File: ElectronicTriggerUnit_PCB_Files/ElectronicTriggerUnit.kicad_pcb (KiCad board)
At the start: 2 copper layers, 59.7 x 50 mm, 50 parts, among them IC1 MCP1407-E_SN, IC2 ATTINY814-SSF, J2 Conn_01x05, J4 Conn_01x04, Q1 LC191PTDT, Q2 LKPT30102B-A01, Q3 78-SQRS140ELP, Q4 LC191PTDT, U1 Gnd, U2 12v, U3 GndMotor, U4 Gnd, U5 12v

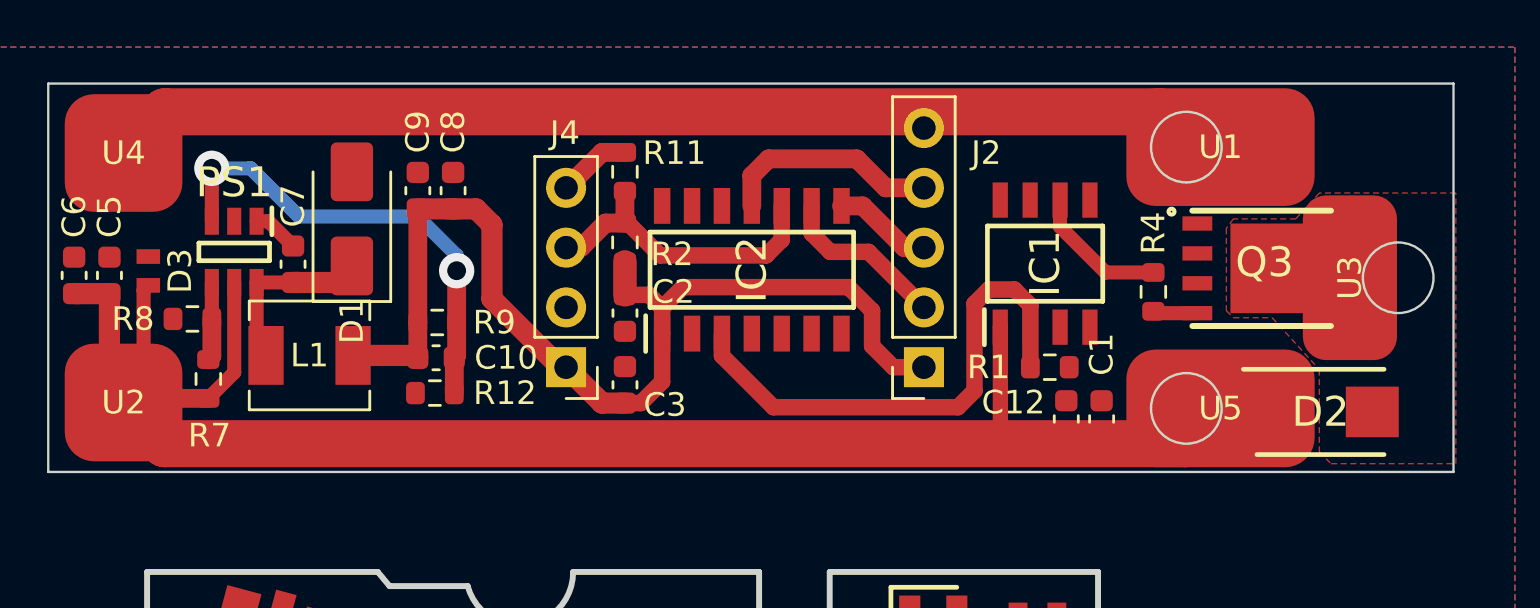
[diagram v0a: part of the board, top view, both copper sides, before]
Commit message: Fixes
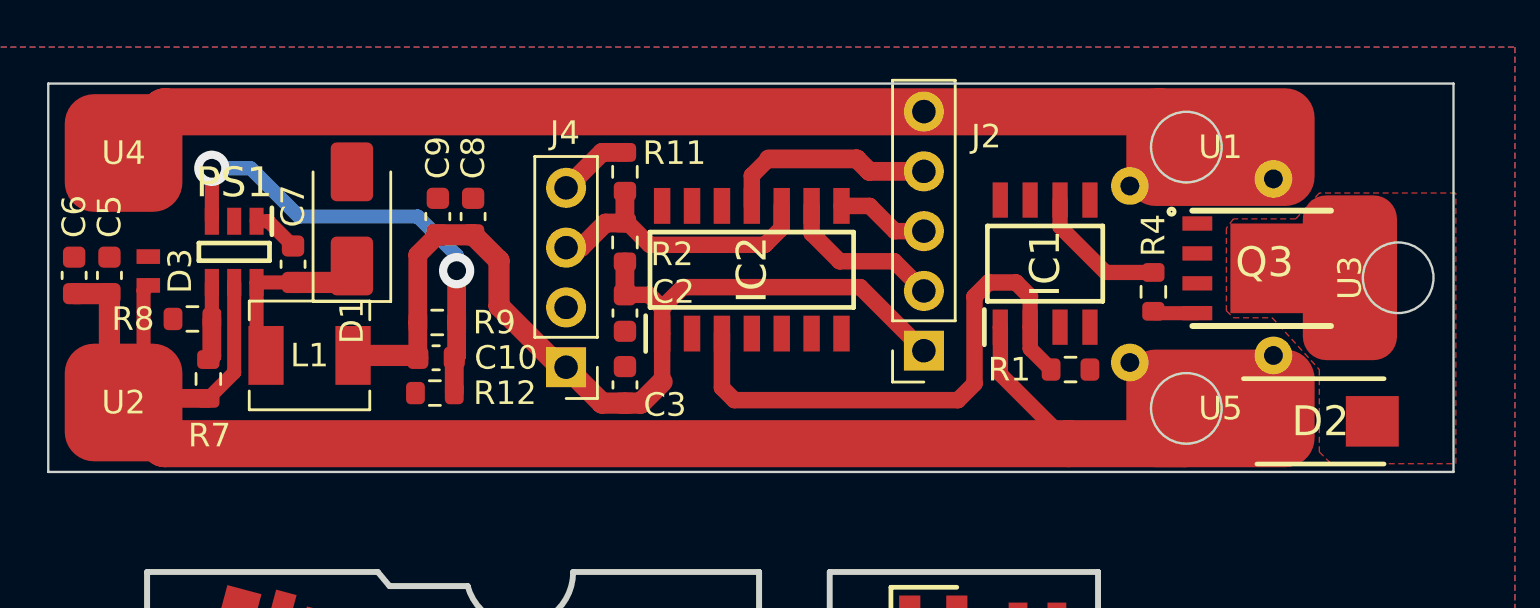
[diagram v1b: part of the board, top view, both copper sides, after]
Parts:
- C1, C12: footprint Capacitor_SMD:C_0603_1608Metric -> Capacitor_THT:C_Axial_L5.1mm_D3.1mm_P7.50mm_Horizontal; moved to B.Cu
- moved C1 9.97 mm to (110.6, 83.4)
- moved C12 9.20 mm to (116.7, 90.6)
- moved C8 1.39 mm to (82.7, 84.7)
- moved C9 1.39 mm to (81.2, 84.7)
- moved R1 0.89 mm to (108.1, 91.2)
- moved J2 0.70 mm to (101.8, 90.4)
- moved D2 0.40 mm to (118.7, 93.4)
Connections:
- LED4 pad 3: GND -> (no net)
- Q2 pad 3: GND -> (no net)
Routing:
- net +3.3V: track 87.2 -> 83.3 mm
- net /NMOS: track 22.1 -> 23.6 mm
- net +12V: track 73.7 -> 74.9 mm
- net /updiRx: track 13.2 -> 12.6 mm

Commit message: Fixes
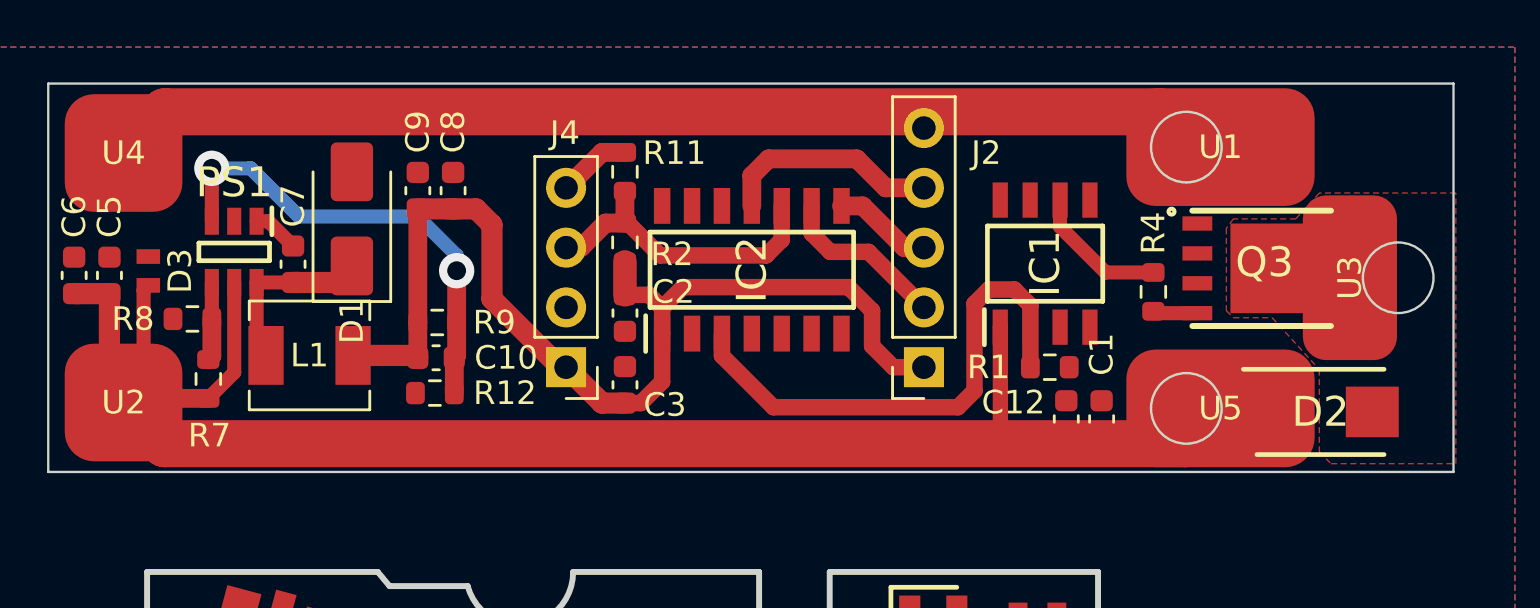
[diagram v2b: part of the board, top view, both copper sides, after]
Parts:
- C1, C12: footprint Capacitor_THT:C_Axial_L5.1mm_D3.1mm_P7.50mm_Horizontal -> Capacitor_SMD:C_0603_1608Metric; moved to F.Cu
- moved C1 9.97 mm to (109.4, 93.3)
- moved C12 9.20 mm to (107.9, 93.3)
- moved C8 1.39 mm to (81.8, 83.6)
- moved C9 1.39 mm to (80.3, 83.6)
- moved R1 0.89 mm to (107.2, 91.1)
- moved J2 0.70 mm to (101.8, 91.1)
- moved D2 0.40 mm to (118.7, 93.0)
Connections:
- LED4 pad 3: (no net) -> GND
- Q2 pad 3: (no net) -> GND
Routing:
- net +3.3V: track 83.3 -> 87.2 mm
- net /NMOS: track 23.6 -> 22.1 mm
- net +12V: track 74.9 -> 73.7 mm
- net /updiRx: track 12.6 -> 13.2 mm
